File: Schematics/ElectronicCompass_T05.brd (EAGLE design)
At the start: 63.2 x 61 mm, 61 parts, among them Q1 FDN360P, Q2 FDN360P, Q3 FDN360P, Q4 FDN360P, U1 ATMEGA32U4, X1 USBSMD, Y1 16MHz

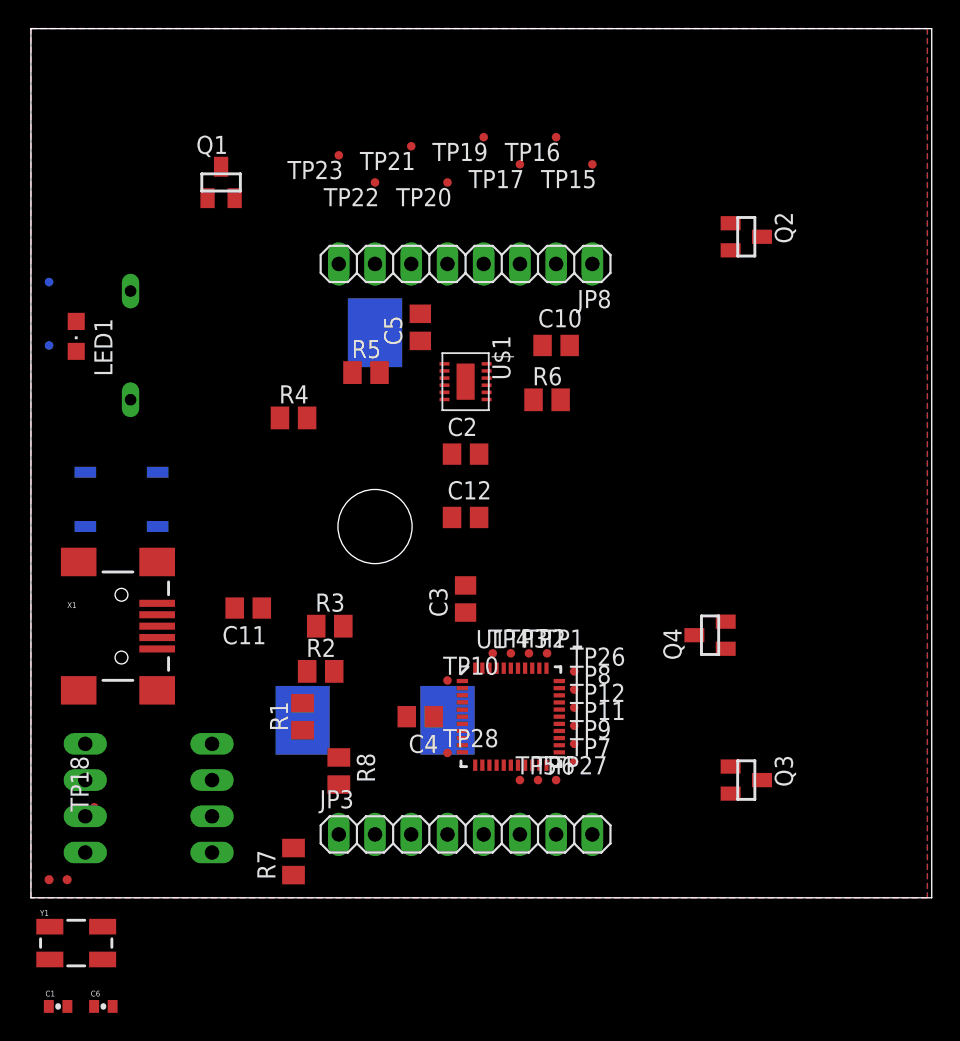
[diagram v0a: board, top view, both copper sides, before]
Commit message: gpio change push
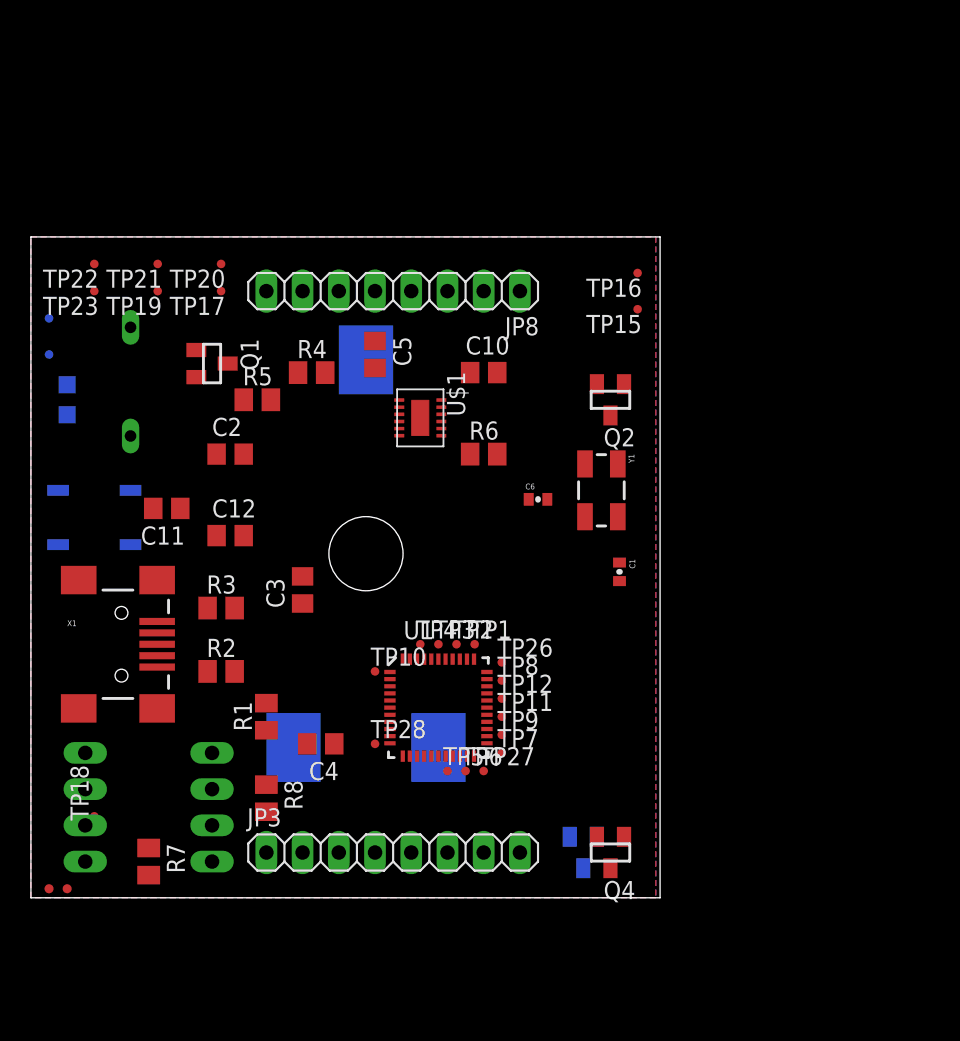
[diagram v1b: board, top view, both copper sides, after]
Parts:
- moved C1 49.8 mm to (41.3, 22.9), turned to 270 degrees
- moved Y1 48.6 mm to (40.0, 28.6), turned to 270 degrees
- moved C6 46.8 mm to (35.6, 27.9)
- moved TP19 25.3 mm to (8.89, 42.5)
- moved TP17 22.8 mm to (13.3, 42.5)
- moved TP22 20.5 mm to (4.45, 44.5)
- moved TP23 19.6 mm to (4.45, 42.5)
- moved TP21 19.6 mm to (8.89, 44.5)
- moved TP20 16.9 mm to (13.3, 44.5)
- moved Q4 16.8 mm to (40.6, 3.17), turned to 180 degrees
- moved C12 16.6 mm to (14.0, 25.4)
- moved C2 16.5 mm to (14.0, 31.1)
- moved Q2 14.9 mm to (40.6, 34.9), turned to 180 degrees
- moved Q1 12.7 mm to (12.7, 37.5), turned to 270 degrees
- moved Q3 12.5 mm to (38.7, 3.17), flipped to the bottom, turned to 180 degrees
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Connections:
- removed net N$2 (its old number): U1.17
- removed net N$26 (its old number): TP12.TP, U1.29
- net D/C: now also U1.28; no longer U1.12
- net GND: now also U$1.P13, U$1.P3
- net N$25: now also U1.12; no longer U1.28
- net N$3: now also TP12.TP, U1.26; no longer U1.16
- net N$4: now also U$1.P1
- net N$41: now also U1.17
- net N$42: now also U1.16
- net RESET: now also U1.29; no longer U1.26
- net VCC: now also U$1.P4, U$1.P5
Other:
- board size 63.2 x 61 mm -> 44.1 x 46.3 mm

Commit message: board layout complete
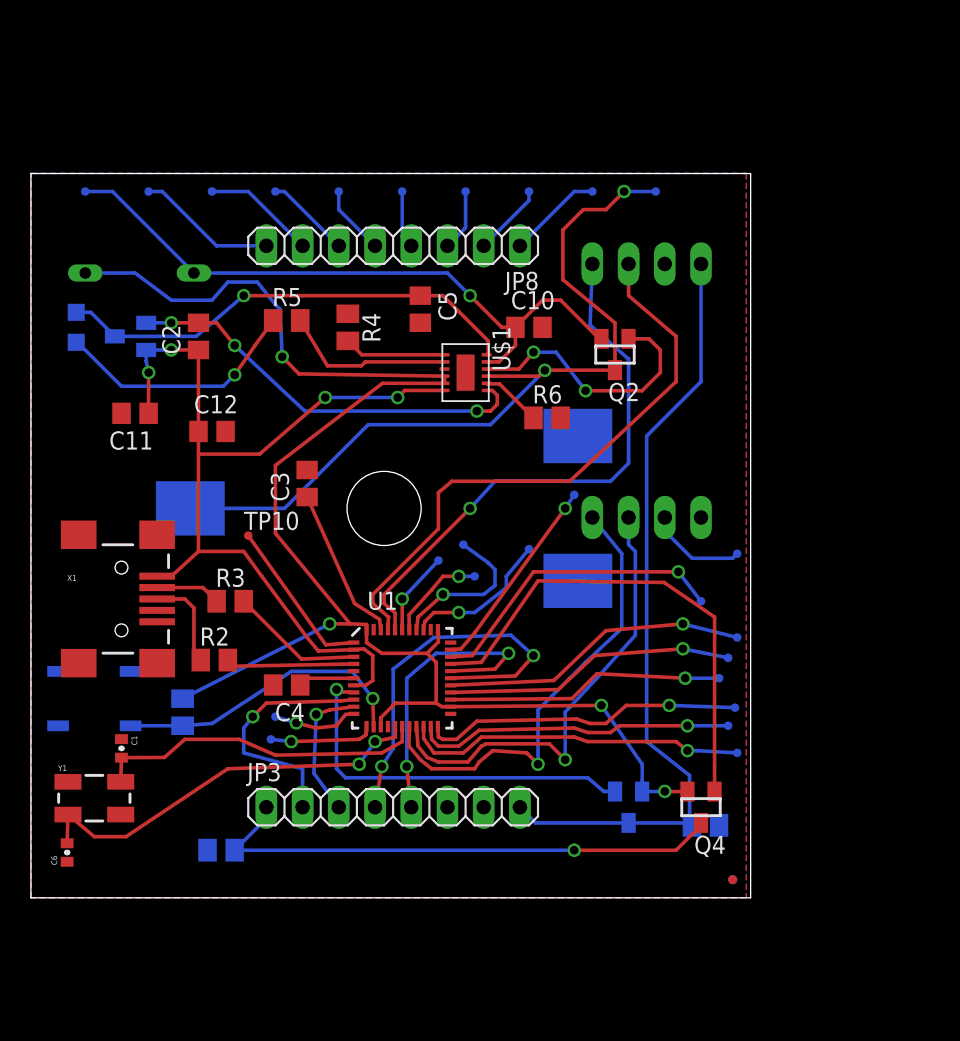
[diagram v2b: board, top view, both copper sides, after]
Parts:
- moved JP2 48.8 mm to (43.2, 44.5), turned to 180 degrees
- moved TP18 48.7 mm to (49.5, 24.1), flipped to the bottom, turned to 270 degrees
- moved JP7 47.9 mm to (49.2, 1.27)
- moved JP6 46.7 mm to (49.2, 1.27), flipped to the bottom
- moved JP1 44.3 mm to (43.2, 26.7), turned to 180 degrees
- moved TP24 44.1 mm to (43.8, 49.5)
- moved Y1 41.6 mm to (4.45, 6.99), turned to 0 degrees
- moved C6 41.3 mm to (2.54, 3.17), turned to 90 degrees
- moved R7 39.1 mm to (47.3, 5.08), flipped to the bottom, turned to 0 degrees
- moved C1 37.1 mm to (6.35, 10.5)
- moved TP5 20.4 mm to (49.5, 10.2), flipped to the bottom
- moved TP6 18.7 mm to (48.9, 12.1), flipped to the bottom
- moved TP17 18.5 mm to (30.5, 49.5), flipped to the bottom
- moved TP19 18.5 mm to (26.0, 49.5), flipped to the bottom
- moved TP27 18.2 mm to (49.4, 13.3), flipped to the bottom
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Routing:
- net VCC: track 0.00 -> 110.7 mm, vias 0 -> 4
- net N$11: track 0.00 -> 63.9 mm, vias 0 -> 4
- net N$5: track 0.00 -> 57.2 mm, vias 0 -> 2
- net VCC': track 0.00 -> 54.8 mm
- net N$36: track 0.00 -> 45.8 mm, vias 0 -> 1
- net INT2: track 0.00 -> 41.5 mm
- net INT1: track 0.00 -> 39.0 mm, vias 0 -> 1
- net LCD_BKLT: track 0.00 -> 37.5 mm, vias 0 -> 1
- net N$26: track 0.00 -> 34.5 mm
- net N$6: track 0.00 -> 33.0 mm, vias 0 -> 1
- net SCL: track 0.00 -> 32.5 mm, vias 0 -> 1
- net SDA: track 0.00 -> 32.2 mm, vias 0 -> 1
- net N$9: track 0.00 -> 28.9 mm, vias 0 -> 3
- net N$42: track 0.00 -> 28.6 mm, vias 0 -> 2
- net D/C: track 0.00 -> 27.6 mm, vias 0 -> 2
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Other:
- board size 44.1 x 46.3 mm -> 50.5 x 50.8 mm

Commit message: push xtal move
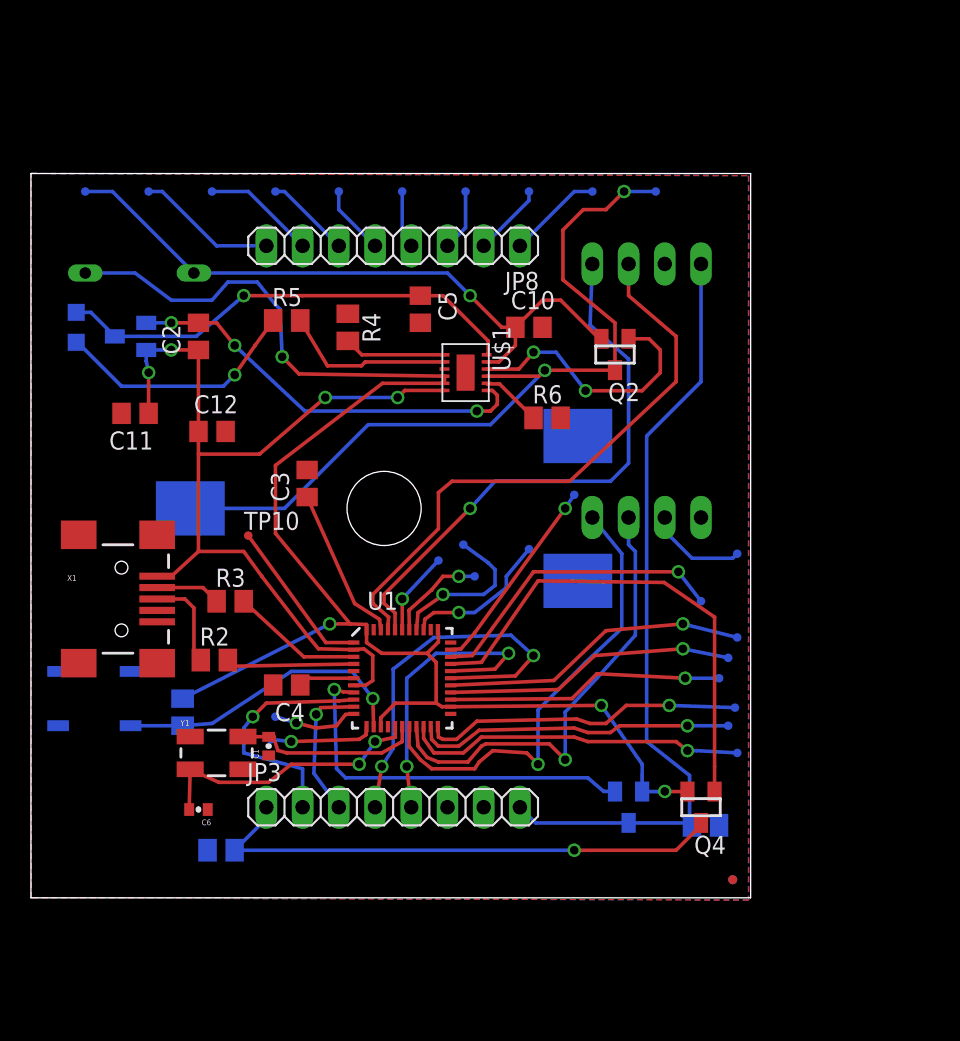
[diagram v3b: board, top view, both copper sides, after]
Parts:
- moved C1 10.3 mm to (16.7, 10.6), turned to 90 degrees
- moved C6 9.69 mm to (11.7, 6.19), turned to 180 degrees
- moved Y1 9.14 mm to (13.0, 10.2)
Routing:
- net N$41: track 23.3 -> 13.1 mm
- net N$42: track 28.6 -> 19.4 mm
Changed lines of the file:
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@@
 <element name="Q4" library="transistor-power" package="SUPER-SOT3" value="FDN360P" x="46.99" y="6.35" rot="R180"/>
 <element name="Q1" library="transistor-power" package="SUPER-SOT3" value="FDN360P" x="6.985" y="39.37" rot="MR270"/>
-<element name="Y1" library="SparkFun" package="CRYSTAL-SMD-5X3" value="16MHz" x="4.445" y="6.985"/>
-<element name="C1" library="SparkFun" package="0402-CAP" value="18pF" x="6.35" y="10.4775" rot="R270"/>
-<element name="C6" library="SparkFun" package="0402-CAP" value="18pF" x="2.54" y="3.175" rot="R90"/>
+<element name="Y1" library="SparkFun" package="CRYSTAL-SMD-5X3" value="16MHz" x="13.0175" y="10.16"/>
+<element name="C1" library="SparkFun" package="0402-CAP" value="18pF" x="16.66875" y="10.63625" rot="R90"/>
+<element name="C6" library="SparkFun" package="0402-CAP" value="18pF" x="11.7475" y="6.19125" rot="R180"/>
 </elements>
 <signals>
@@
 <polygon width="0.4064" layer="16">
 <vertex x="0" y="50.8"/>
-<vertex x="50.165" y="50.8"/>
-<vertex x="50.165" y="0"/>
+<vertex x="50.32375" y="50.64125"/>
+<vertex x="50.32375" y="-0.15875"/>
 <vertex x="0" y="0"/>
 </polygon>
 <polygon width="0.4064" layer="1">
 <vertex x="0" y="50.8"/>
-<vertex x="50.165" y="50.8"/>
-<vertex x="50.165" y="0"/>
+<vertex x="50.32375" y="50.64125"/>
+<vertex x="50.32375" y="-0.15875"/>
 <vertex x="0" y="0"/>
 </polygon>
@@
 <contactref element="U1" pad="3"/>
 <contactref element="R3" pad="2"/>
-<wire x1="22.635" y1="16.89875" x2="18.97625" y2="16.74" width="0.254" layer="1"/>
-<wire x1="18.97625" y1="16.74" x2="14.92" y2="20.79625" width="0.254" layer="1"/>
+<wire x1="22.635" y1="16.89875" x2="19.135" y2="16.89875" width="0.254" layer="1"/>
+<wire x1="19.135" y1="16.89875" x2="14.92" y2="20.79625" width="0.254" layer="1"/>
 </signal>
 <signal name="N$12">
@@
 <contactref element="U1" pad="36"/>
 <contactref element="TP1" pad="TP"/>
-<wire x1="27.535" y1="18.79875" x2="27.6225" y2="19.3675" width="0.254" layer="1"/>
-<wire x1="27.6225" y1="19.3675" x2="28.2575" y2="20.0025" width="0.254" layer="1"/>
+<wire x1="27.535" y1="18.79875" x2="27.6225" y2="19.52625" width="0.254" layer="1"/>
+<wire x1="27.6225" y1="19.52625" x2="28.2575" y2="20.0025" width="0.254" layer="1"/>
 <wire x1="28.2575" y1="20.0025" x2="30.00375" y2="20.0025" width="0.254" layer="1"/>
 <via x="30.00375" y="20.0025" extent="1-16" drill="0.6"/>
@@
 <contactref element="U1" pad="37"/>
 <contactref element="TP2" pad="TP"/>
-<wire x1="27.035" y1="18.79875" x2="27.14625" y2="19.685" width="0.254" layer="1"/>
-<wire x1="27.14625" y1="19.685" x2="28.73375" y2="21.11375" width="0.254" layer="1"/>
+<wire x1="27.035" y1="18.79875" x2="27.14625" y2="20.0025" width="0.254" layer="1"/>
+<wire x1="27.14625" y1="20.0025" x2="28.73375" y2="21.11375" width="0.254" layer="1"/>
 <wire x1="28.73375" y1="21.11375" x2="28.8925" y2="21.2725" width="0.254" layer="1"/>
 <via x="28.8925" y="21.2725" extent="1-16" drill="0.6"/>
@@
 <contactref element="U1" pad="38"/>
 <contactref element="TP3" pad="TP"/>
-<wire x1="26.535" y1="18.79875" x2="26.51125" y2="19.84375" width="0.254" layer="1"/>
-<wire x1="26.51125" y1="19.84375" x2="28.09875" y2="21.59" width="0.254" layer="1"/>
+<wire x1="26.535" y1="18.79875" x2="26.51125" y2="20.16125" width="0.254" layer="1"/>
+<wire x1="26.51125" y1="20.16125" x2="28.09875" y2="21.59" width="0.254" layer="1"/>
 <wire x1="28.09875" y1="21.59" x2="28.8925" y2="22.5425" width="0.254" layer="1"/>
 <wire x1="28.8925" y1="22.5425" x2="30.00375" y2="22.5425" width="0.254" layer="1"/>
@@
 <contactref element="U1" pad="1"/>
 <contactref element="TP10" pad="TP"/>
-<wire x1="22.635" y1="17.89875" x2="20.6775" y2="17.74" width="0.254" layer="1"/>
-<wire x1="20.6775" y1="17.74" x2="15.24" y2="25.4" width="0.254" layer="1"/>
+<wire x1="22.635" y1="17.89875" x2="20.6775" y2="17.89875" width="0.254" layer="1"/>
+<wire x1="20.6775" y1="17.89875" x2="15.24" y2="25.4" width="0.254" layer="1"/>
 </signal>
 <signal name="INT1">
@@
 <wire x1="19.05" y1="9.04875" x2="14.9225" y2="10.16" width="0.254" layer="16"/>
 <wire x1="14.9225" y1="10.16" x2="14.9225" y2="11.90625" width="0.254" layer="16"/>
-<wire x1="22.635" y1="13.89875" x2="21.74875" y2="13.81125" width="0.254" layer="1"/>
-<wire x1="21.74875" y1="13.81125" x2="16.51" y2="13.6525" width="0.254" layer="1"/>
+<wire x1="22.635" y1="13.89875" x2="21.59" y2="13.81125" width="0.254" layer="1"/>
+<wire x1="21.59" y1="13.81125" x2="16.51" y2="13.6525" width="0.254" layer="1"/>
 <wire x1="16.51" y1="13.6525" x2="15.5575" y2="12.7" width="0.254" layer="1"/>
 <wire x1="14.9225" y1="11.90625" x2="15.5575" y2="12.7" width="0.254" layer="16"/>
@@
 <wire x1="21.59" y1="6.35" x2="19.84375" y2="8.73125" width="0.254" layer="16"/>
 <wire x1="19.84375" y1="8.73125" x2="20.0025" y2="12.85875" width="0.254" layer="16"/>
-<wire x1="22.635" y1="13.39875" x2="20.955" y2="13.17625" width="0.254" layer="1"/>
-<wire x1="20.955" y1="13.17625" x2="20.0025" y2="12.85875" width="0.254" layer="1"/>
+<wire x1="22.635" y1="13.39875" x2="20.32" y2="13.335" width="0.254" layer="1"/>
+<wire x1="20.32" y1="13.335" x2="20.0025" y2="12.85875" width="0.254" layer="1"/>
 <via x="20.0025" y="12.85875" extent="1-16" drill="0.6"/>
 </signal>
@@
 <wire x1="11.7475" y1="24.28875" x2="14.9225" y2="24.28875" width="0.254" layer="1"/>
 <wire x1="14.9225" y1="24.28875" x2="16.1925" y2="22.5425" width="0.254" layer="1"/>
-<wire x1="16.1925" y1="22.5425" x2="19.3675" y2="18.25625" width="0.254" layer="1"/>
-<wire x1="19.3675" y1="18.25625" x2="20.16125" y2="17.30375" width="0.254" layer="1"/>
+<wire x1="16.1925" y1="22.5425" x2="19.3675" y2="18.415" width="0.254" layer="1"/>
+<wire x1="19.3675" y1="18.415" x2="20.16125" y2="17.4625" width="0.254" layer="1"/>
 <wire x1="22.635" y1="14.89875" x2="23.47125" y2="14.89875" width="0.254" layer="1"/>
 <wire x1="23.47125" y1="14.89875" x2="23.97125" y2="15.24" width="0.254" layer="1"/>
@@
 <via x="25.7175" y="35.08375" extent="1-16" drill="0.6"/>
 <wire x1="23.97125" y1="16.98625" x2="23.33625" y2="17.4625" width="0.254" layer="1"/>
-<wire x1="20.16125" y1="17.30375" x2="22.635" y2="17.39875" width="0.254" layer="1"/>
+<wire x1="20.16125" y1="17.4625" x2="22.635" y2="17.39875" width="0.254" layer="1"/>
 <wire x1="23.33625" y1="17.4625" x2="22.635" y2="17.39875" width="0.254" layer="1"/>
 <wire x1="11.75" y1="32.7025" x2="11.7475" y2="31.115" width="0" layer="19" extent="1-1"/>
@@
 <wire x1="39.0525" y1="8.41375" x2="22.06625" y2="8.41375" width="0.254" layer="16"/>
 <wire x1="22.06625" y1="8.41375" x2="21.43125" y2="9.04875" width="0.254" layer="16"/>
-<wire x1="21.43125" y1="9.04875" x2="21.43125" y2="14.605" width="0.254" layer="16"/>
+<wire x1="21.43125" y1="9.04875" x2="21.2725" y2="14.605" width="0.254" layer="16"/>
 <wire x1="22.635" y1="14.39875" x2="21.9075" y2="14.44625" width="0.254" layer="1"/>
-<wire x1="21.9075" y1="14.44625" x2="21.43125" y2="14.605" width="0.254" layer="1"/>
-<via x="21.43125" y="14.605" extent="1-16" drill="0.6"/>
+<wire x1="21.9075" y1="14.44625" x2="21.2725" y2="14.605" width="0.254" layer="1"/>
+<via x="21.2725" y="14.605" extent="1-16" drill="0.6"/>
 </signal>
 <signal name="N$39">
@@
 <contactref element="Y1" pad="3"/>
 <contactref element="U1" pad="17"/>
-<wire x1="6.295" y1="8.135" x2="6.35" y2="9.8275" width="0.254" layer="1"/>
-<wire x1="6.35" y1="9.8275" x2="9.36625" y2="9.8425" width="0.254" layer="1"/>
-<wire x1="9.36625" y1="9.8425" x2="10.795" y2="11.1125" width="0.254" layer="1"/>
-<wire x1="10.795" y1="11.1125" x2="14.605" y2="11.1125" width="0.254" layer="1"/>
-<wire x1="14.605" y1="11.1125" x2="17.145" y2="10.00125" width="0.254" layer="1"/>
-<wire x1="17.145" y1="10.00125" x2="24.60625" y2="10.16" width="0.254" layer="1"/>
+<wire x1="14.8675" y1="11.31" x2="16.66875" y2="11.28625" width="0.254" layer="1"/>
 <wire x1="24.60625" y1="10.16" x2="26.035" y2="10.95375" width="0.254" layer="1"/>
 <wire x1="26.035" y1="10.95375" x2="26.035" y2="11.99875" width="0.254" layer="1"/>
+<wire x1="16.66875" y1="11.28625" x2="17.00125" y2="11.28625" width="0.4064" layer="1"/>
+<wire x1="17.00125" y1="11.28625" x2="17.31875" y2="10.33375" width="0.254" layer="1"/>
+<wire x1="17.31875" y1="10.33375" x2="17.93875" y2="10.16" width="0.254" layer="1"/>
+<wire x1="17.93875" y1="10.16" x2="24.60625" y2="10.16" width="0.254" layer="1"/>
 </signal>
 <signal name="N$42">
@@
 <contactref element="C6" pad="2"/>
 <contactref element="U1" pad="16"/>
-<wire x1="2.595" y1="5.835" x2="2.54" y2="3.825" width="0.254" layer="1"/>
-<wire x1="2.595" y1="5.835" x2="4.445" y2="4.28625" width="0.254" layer="1"/>
-<wire x1="4.445" y1="4.28625" x2="6.6675" y2="4.28625" width="0.254" layer="1"/>
-<wire x1="6.6675" y1="4.28625" x2="13.81125" y2="9.04875" width="0.254" layer="1"/>
-<wire x1="13.81125" y1="9.04875" x2="23.01875" y2="9.36625" width="0.254" layer="1"/>
+<wire x1="11.1675" y1="9.01" x2="11.0975" y2="6.19125" width="0.254" layer="1"/>
+<wire x1="11.1675" y1="9.01" x2="13.17625" y2="8.09625" width="0.254" layer="1"/>
+<wire x1="13.17625" y1="8.09625" x2="16.66875" y2="8.09625" width="0.254" layer="1"/>
+<wire x1="16.66875" y1="8.09625" x2="18.25625" y2="9.36625" width="0.254" layer="1"/>
 <wire x1="25.535" y1="11.99875" x2="25.55875" y2="11.27125" width="0.254" layer="1"/>
 <wire x1="25.55875" y1="11.27125" x2="24.13" y2="10.95375" width="0.254" layer="1"/>
@@
 <via x="24.13" y="10.95375" extent="1-16" drill="0.6"/>
 <via x="23.01875" y="9.36625" extent="1-16" drill="0.6"/>
+<wire x1="18.25625" y1="9.36625" x2="23.01875" y2="9.36625" width="0.254" layer="1"/>
 </signal>
 <signal name="N$2">
